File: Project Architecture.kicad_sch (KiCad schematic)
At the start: 40 parts, among them J1 USB4105-GF-A, Q1 PT334-6C, U1 LM393, U2 USBLC6-2SC6, U3 FT231XS-U

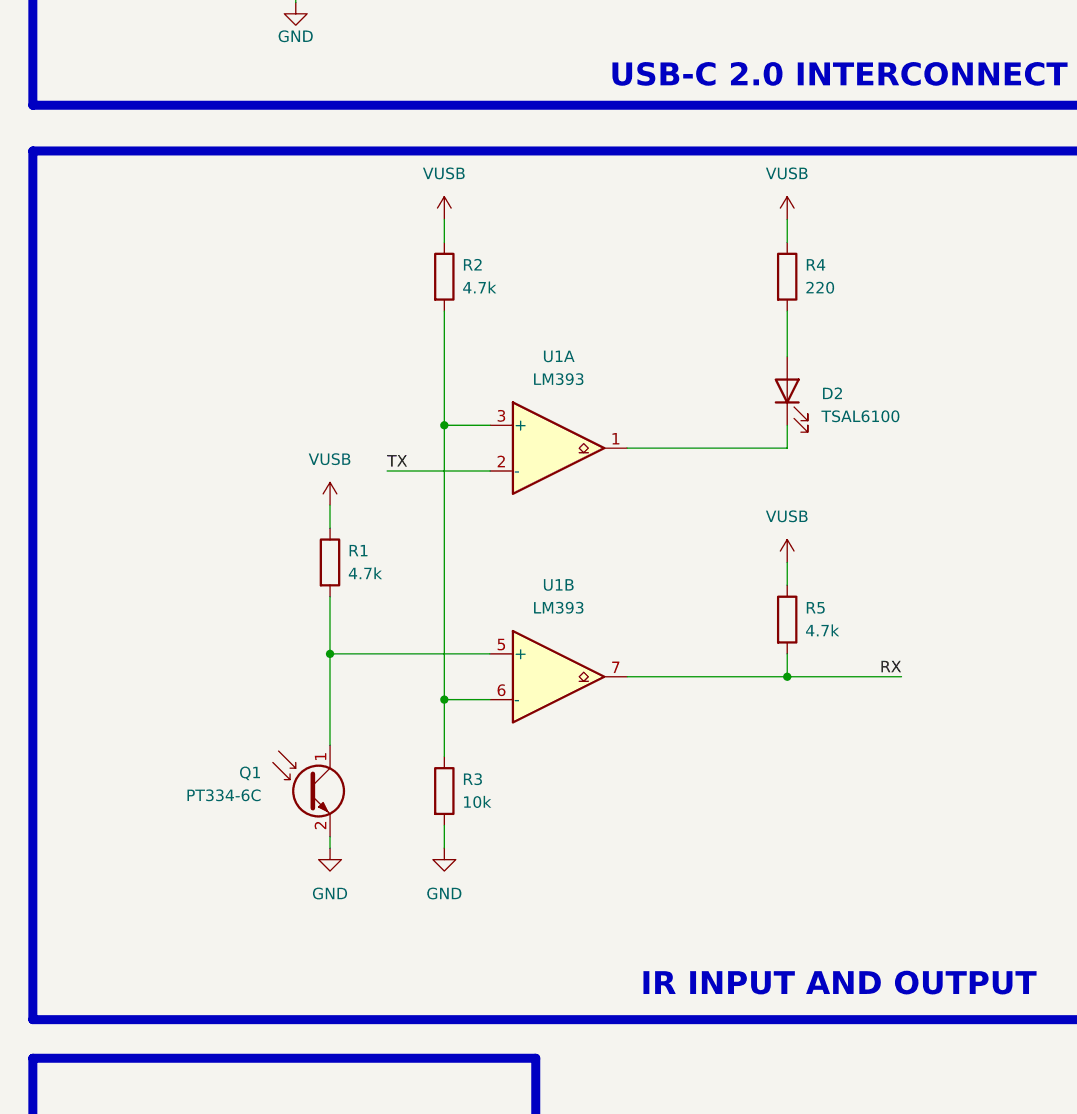
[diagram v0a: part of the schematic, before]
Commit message: chore: snapshot project before Boardwright migration
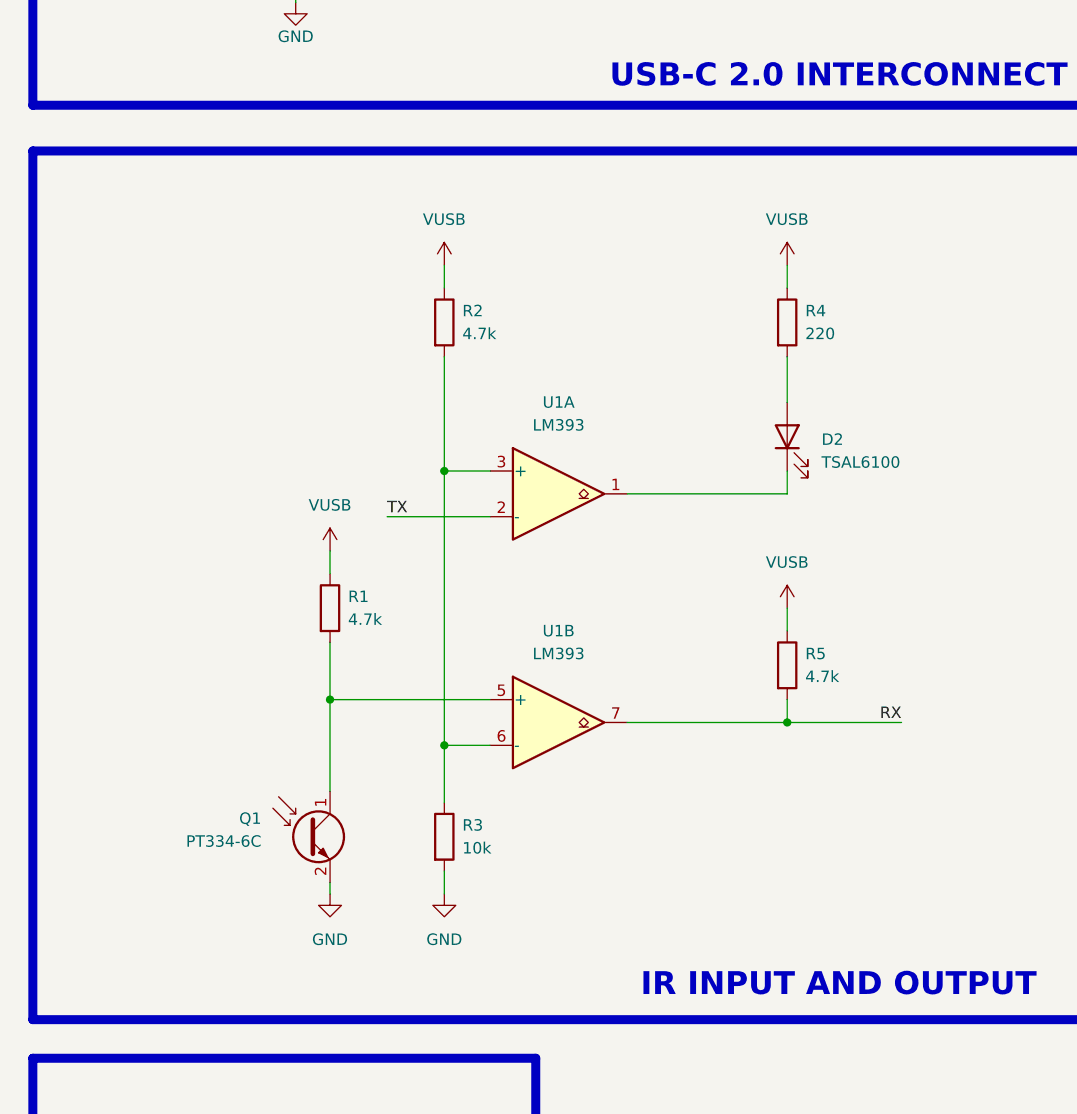
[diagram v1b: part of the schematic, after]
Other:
- moved on the sheet: D2, Q1, R1, R2, R3, R4, R5, U1A, U1B
